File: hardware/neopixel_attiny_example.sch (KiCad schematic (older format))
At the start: 19 parts, among them J1 AVR-ISP-6, U1 ATtiny13A-PU

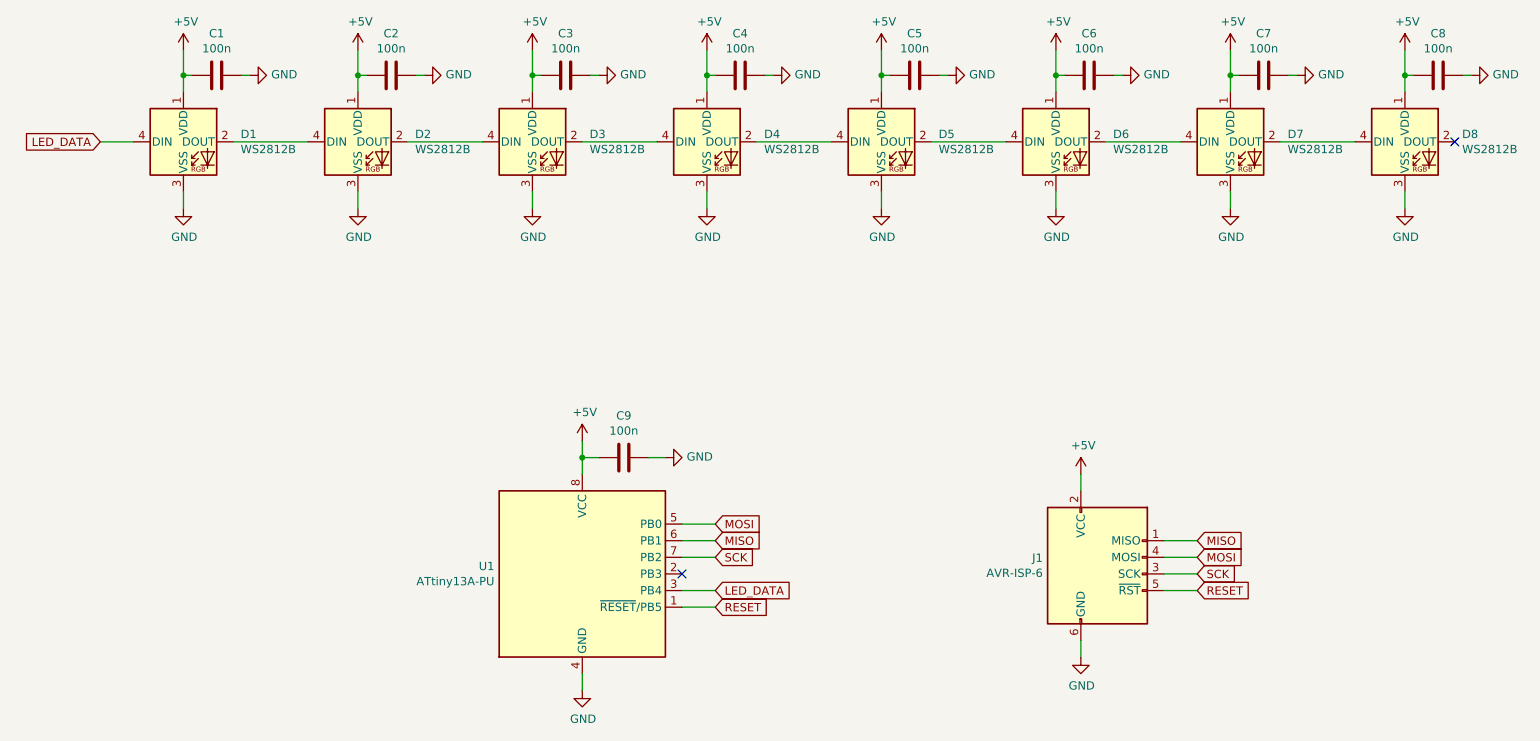
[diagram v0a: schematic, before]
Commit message: added firmware for attiny13
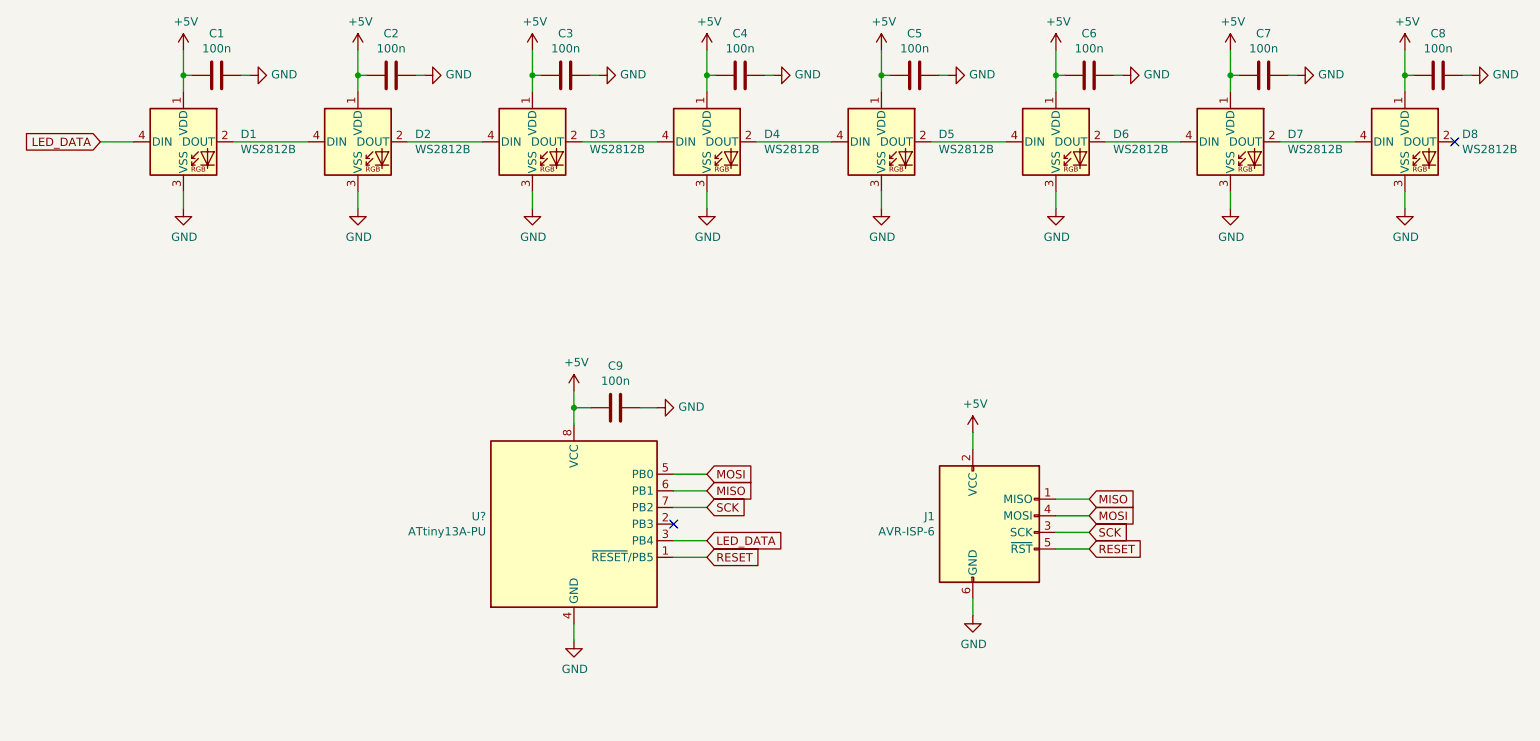
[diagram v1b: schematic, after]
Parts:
- removed U1: ATtiny13A-PU, Package_DIP:DIP-8_W7.62mm, symbol MCU_Microchip_ATtiny:ATtiny13A-PU
- added U?: ATtiny13A-PU, Package_DIP:DIP-8_W7.62mm, symbol MCU_Microchip_ATtiny:ATtiny13A-PU
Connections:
- net +5V: now also U?.8 (VCC)
- net GND: now also U?.4 (GND)
- net LED_DATA: now also U?.3 (PB4)
- net MISO: now also U?.6 (PB1)
- net MOSI: now also U?.5 (PB0)
- net RESET: now also U?.1 (~RESET~/PB5)
- net SCK: now also U?.7 (PB2)
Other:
- moved on the sheet: C9, J1
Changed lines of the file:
@@
 Sheet 1 1
 Title "Example for W2812B (Neopixel)"
-Date "2020-11-09"
+Date "2020-11-23"
 Rev "V1.0.0"
 Comp ""
@@
 	3100 2350 3100 2450
 $Comp
-L MCU_Microchip_ATtiny:ATtiny13A-PU U1
-U 1 1 5FAC0E98
-P 4450 4650
-F 0 "U1" H 3921 4696 50  0000 R CNN
-F 1 "ATtiny13A-PU" H 3921 4605 50  0000 R CNN
-F 2 "Package_DIP:DIP-8_W7.62mm" H 4450 4650 50  0001 C CIN
-F 3 "http://ww1.microchip.com/downloads/en/DeviceDoc/doc8126.pdf" H 4450 4650 50  0001 C CNN
-	1    4450 4650
-	1    0    0    -1
-$EndComp
-$Comp
 L power:+5V #PWR0125
 U 1 1 5FAC421F
-P 4450 3850
-F 0 "#PWR0125" H 4450 3700 50  0001 C CNN
-F 1 "+5V" H 4465 4023 50  0000 C CNN
-F 2 "" H 4450 3850 50  0001 C CNN
-F 3 "" H 4450 3850 50  0001 C CNN
-	1    4450 3850
-	1    0    0    -1
-$EndComp
-Wire Wire Line
-	4450 3850 4450 3950
+P 4400 3550
+F 0 "#PWR0125" H 4400 3400 50  0001 C CNN
+F 1 "+5V" H 4415 3723 50  0000 C CNN
+F 2 "" H 4400 3550 50  0001 C CNN
+F 3 "" H 4400 3550 50  0001 C CNN
+	1    4400 3550
+	1    0    0    -1
+$EndComp
+Wire Wire Line
+	4400 3550 4400 3650
 $Comp
 L Device:C C9
 U 1 1 5FAC5C9E
-P 4700 3950
-F 0 "C9" V 4448 3950 50  0000 C CNN
-F 1 "100n" V 4539 3950 50  0000 C CNN
-F 2 "" H 4738 3800 50  0001 C CNN
-F 3 "~" H 4700 3950 50  0001 C CNN
-	1    4700 3950
+P 4650 3650
+F 0 "C9" V 4398 3650 50  0000 C CNN
+F 1 "100n" V 4489 3650 50  0000 C CNN
+F 2 "" H 4688 3500 50  0001 C CNN
+F 3 "~" H 4650 3650 50  0001 C CNN
+	1    4650 3650
 	0    1    1    0
 $EndComp
@@
 L power:GND #PWR0126
 U 1 1 5FAC6E3D
-P 4950 3950
-F 0 "#PWR0126" H 4950 3700 50  0001 C CNN
-F 1 "GND" V 4955 3822 50  0000 R CNN
-F 2 "" H 4950 3950 50  0001 C CNN
-F 3 "" H 4950 3950 50  0001 C CNN
-	1    4950 3950
-	0    -1   -1   0
-$EndComp
-Wire Wire Line
-	4550 3950 4450 3950
-Connection ~ 4450 3950
-Wire Wire Line
-	4450 3950 4450 4050
-Wire Wire Line
-	4850 3950 4950 3950
+P 4900 3650
+F 0 "#PWR0126" H 4900 3400 50  0001 C CNN
+F 1 "GND" V 4905 3522 50  0000 R CNN
+F 2 "" H 4900 3650 50  0001 C CNN
+F 3 "" H 4900 3650 50  0001 C CNN
+	1    4900 3650
+	0    -1   -1   0
+$EndComp
+Wire Wire Line
+	4500 3650 4400 3650
+Connection ~ 4400 3650
+Wire Wire Line
+	4400 3650 4400 3750
+Wire Wire Line
+	4800 3650 4900 3650
 $Comp
 L power:GND #PWR0127
 U 1 1 5FAC8CEE
-P 4450 5350
-F 0 "#PWR0127" H 4450 5100 50  0001 C CNN
-F 1 "GND" H 4455 5177 50  0000 C CNN
-F 2 "" H 4450 5350 50  0001 C CNN
-F 3 "" H 4450 5350 50  0001 C CNN
-	1    4450 5350
-	1    0    0    -1
-$EndComp
-Wire Wire Line
-	4450 5250 4450 5350
-Text GLabel 5250 4750 2    50   Input ~ 0
+P 4400 5050
+F 0 "#PWR0127" H 4400 4800 50  0001 C CNN
+F 1 "GND" H 4405 4877 50  0000 C CNN
+F 2 "" H 4400 5050 50  0001 C CNN
+F 3 "" H 4400 5050 50  0001 C CNN
+	1    4400 5050
+	1    0    0    -1
+$EndComp
+Wire Wire Line
+	4400 4950 4400 5050
+Text GLabel 5200 4450 2    50   Input ~ 0
 LED_DATA
 Wire Wire Line
-	5050 4350 5250 4350
-Text GLabel 5250 4850 2    50   Input ~ 0
+	5000 4050 5200 4050
+Text GLabel 5200 4550 2    50   Input ~ 0
 RESET
-Text GLabel 5250 4450 2    50   Input ~ 0
+Text GLabel 5200 4150 2    50   Input ~ 0
 MISO
-Text GLabel 5250 4550 2    50   Input ~ 0
+Text GLabel 5200 4250 2    50   Input ~ 0
 SCK
-Text GLabel 5250 4350 2    50   Input ~ 0
+Text GLabel 5200 4050 2    50   Input ~ 0
 MOSI
 Wire Wire Line
-	5050 4450 5250 4450
-Wire Wire Line
-	5050 4550 5250 4550
-Wire Wire Line
-	5050 4750 5250 4750
-Wire Wire Line
-	5050 4850 5250 4850
-NoConn ~ 5050 4650
+	5000 4150 5200 4150
+Wire Wire Line
+	5000 4250 5200 4250
+Wire Wire Line
+	5000 4450 5200 4450
+Wire Wire Line
+	5000 4550 5200 4550
 $Comp
 L Connector:AVR-ISP-6 J1
 U 1 1 5FADB754
-P 7550 4650
-F 0 "J1" H 7221 4746 50  0000 R CNN
-F 1 "AVR-ISP-6" H 7221 4655 50  0000 R CNN
-F 2 "" V 7300 4700 50  0001 C CNN
-F 3 " ~" H 6275 4100 50  0001 C CNN
-	1    7550 4650
+P 6900 4400
+F 0 "J1" H 6571 4496 50  0000 R CNN
+F 1 "AVR-ISP-6" H 6571 4405 50  0000 R CNN
+F 2 "" V 6650 4450 50  0001 C CNN
+F 3 " ~" H 5625 3850 50  0001 C CNN
+	1    6900 4400
 	1    0    0    -1
 $EndComp
@@
 L power:GND #PWR0128
 U 1 1 5FAE12B7
-P 7450 5150
-F 0 "#PWR0128" H 7450 4900 50  0001 C CNN
-F 1 "GND" H 7455 4977 50  0000 C CNN
-F 2 "" H 7450 5150 50  0001 C CNN
-F 3 "" H 7450 5150 50  0001 C CNN
-	1    7450 5150
-	1    0    0    -1
-$EndComp
-Wire Wire Line
-	7450 5050 7450 5150
+P 6800 4900
+F 0 "#PWR0128" H 6800 4650 50  0001 C CNN
+F 1 "GND" H 6805 4727 50  0000 C CNN
+F 2 "" H 6800 4900 50  0001 C CNN
+F 3 "" H 6800 4900 50  0001 C CNN
+	1    6800 4900
+	1    0    0    -1
+$EndComp
+Wire Wire Line
+	6800 4800 6800 4900
 $Comp
 L power:+5V #PWR0129
 U 1 1 5FAE28D2
-P 7450 4050
-F 0 "#PWR0129" H 7450 3900 50  0001 C CNN
-F 1 "+5V" H 7465 4223 50  0000 C CNN
-F 2 "" H 7450 4050 50  0001 C CNN
-F 3 "" H 7450 4050 50  0001 C CNN
-	1    7450 4050
-	1    0    0    -1
-$EndComp
-Wire Wire Line
-	7450 4050 7450 4150
-Text GLabel 8150 4550 2    50   Input ~ 0
+P 6800 3800
+F 0 "#PWR0129" H 6800 3650 50  0001 C CNN
+F 1 "+5V" H 6815 3973 50  0000 C CNN
+F 2 "" H 6800 3800 50  0001 C CNN
+F 3 "" H 6800 3800 50  0001 C CNN
+	1    6800 3800
+	1    0    0    -1
+$EndComp
+Wire Wire Line
+	6800 3800 6800 3900
+Text GLabel 7500 4300 2    50   Input ~ 0
 MOSI
-Text GLabel 8150 4450 2    50   Input ~ 0
+Text GLabel 7500 4400 2    50   Input ~ 0
+SCK
+Text GLabel 7500 4500 2    50   Input ~ 0
+RESET
+Wire Wire Line
+	7300 4300 7500 4300
+Wire Wire Line
+	7300 4400 7500 4400
+Wire Wire Line
+	7300 4500 7500 4500
+$Comp
+L MCU_Microchip_ATtiny:ATtiny13A-PU U?
+U 1 1 5FBAC5DD
+P 4400 4350
+F 0 "U?" H 3871 4396 50  0000 R CNN
+F 1 "ATtiny13A-PU" H 3871 4305 50  0000 R CNN
+F 2 "Package_DIP:DIP-8_W7.62mm" H 4400 4350 50  0001 C CIN
+F 3 "http://ww1.microchip.com/downloads/en/DeviceDoc/doc8126.pdf" H 4400 4350 50  0001 C CNN
+	1    4400 4350
+	1    0    0    -1
+$EndComp
+Wire Wire Line
+	7300 4200 7500 4200
+Text GLabel 7500 4200 2    50   Input ~ 0
 MISO
-Text GLabel 8150 4650 2    50   Input ~ 0
-SCK
-Text GLabel 8150 4750 2    50   Input ~ 0
-RESET
-Wire Wire Line
-	7950 4450 8150 4450
-Wire Wire Line
-	7950 4550 8150 4550
-Wire Wire Line
-	7950 4650 8150 4650
-Wire Wire Line
-	7950 4750 8150 4750
+NoConn ~ 5000 4350
 $EndSCHEMATC
